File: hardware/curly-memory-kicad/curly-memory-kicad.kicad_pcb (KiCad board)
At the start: 4 copper layers, 30 x 100 mm, 84 parts, among them J101 Conn_01x06, J102 Conn_01x05, J103 Conn_01x05, J104 Conn_01x05, J105 Conn_01x05, J106 Conn_01x05, J401 Conn_02x05_Odd_Even, U101 MCP3008-I/SL, U102 ESP32-WROOM-32, U103 MCP4822-E/SN, U104 MCP4822-E/SN, U105 MCP42010-E/SL, U106 MCP42010-E/SL, U201 MCP6004, U301 MCP6004, U401 NCP1117-5.0_SOT223, U402 NCP1117-3.3_SOT223

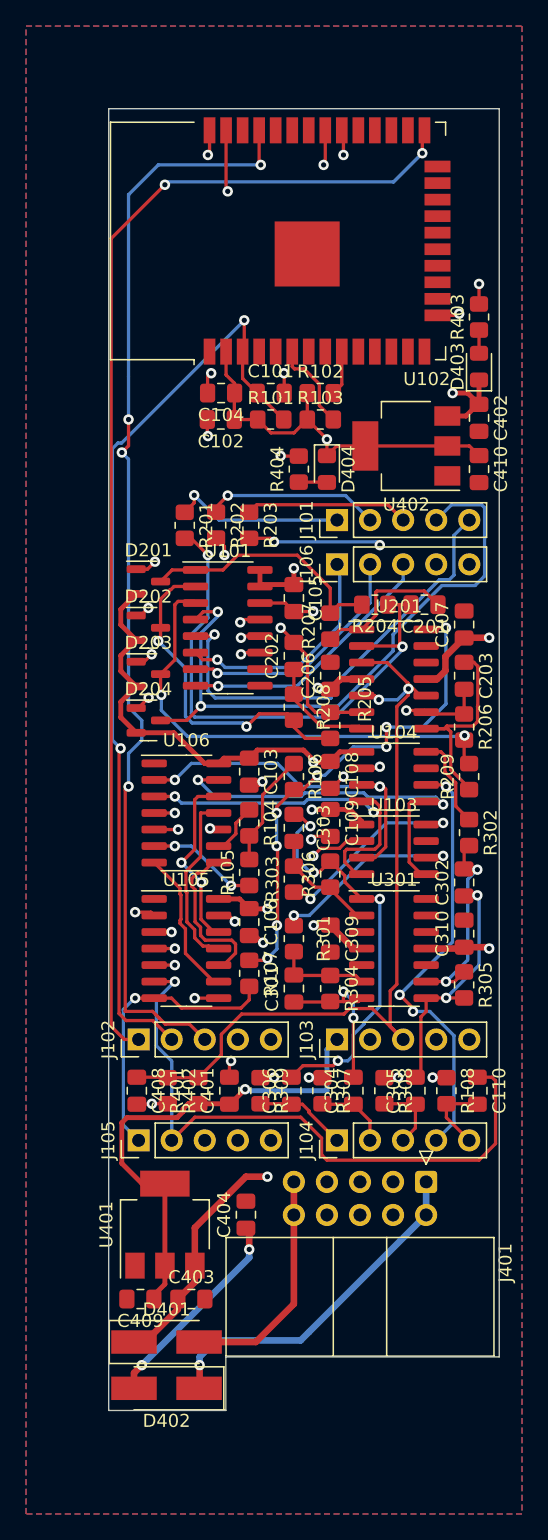
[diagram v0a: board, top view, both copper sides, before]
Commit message: more pcb tracked- again
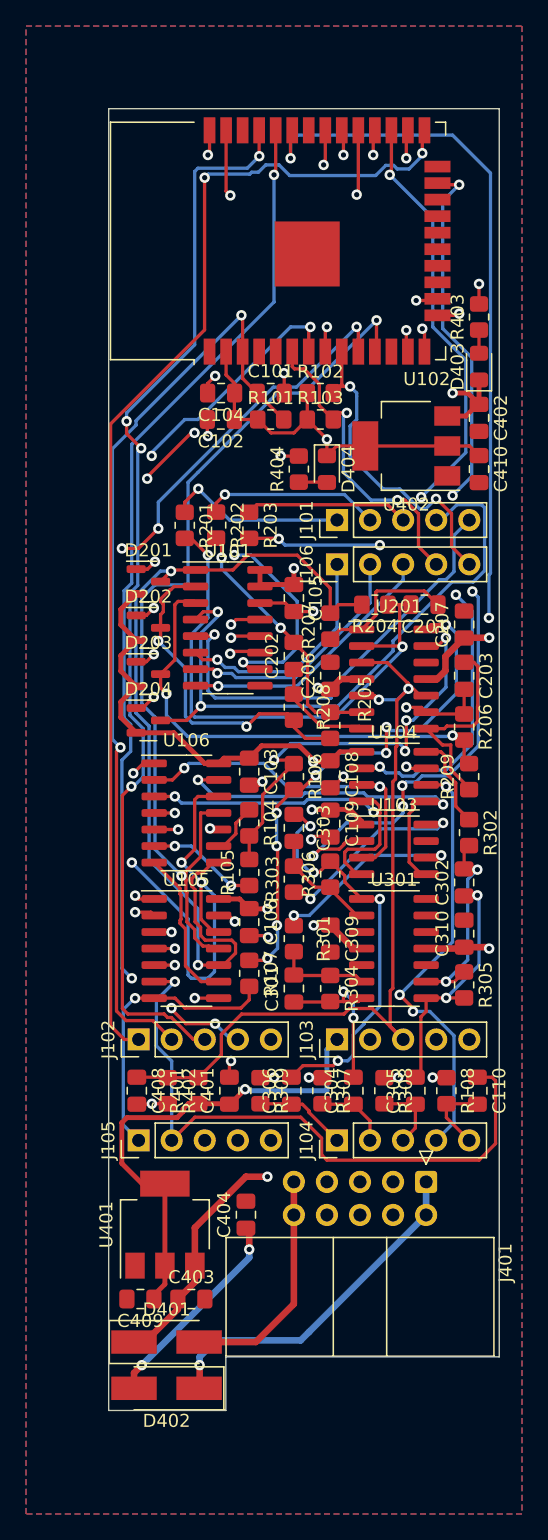
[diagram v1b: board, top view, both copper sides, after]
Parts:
- moved C109 0.05 mm to (17.0, 54.9)
- moved C108 0.05 mm to (17.0, 51.1)
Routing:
- net Net-(J103-Pad5): track 0.00 -> 87.9 mm, vias 0 -> 2
- net /PROG_RX: track 0.00 -> 81.2 mm, vias 0 -> 4
- net /SPI3_CS_1: track 0.00 -> 78.5 mm, vias 0 -> 2
- net /LEDS: track 0.00 -> 77.4 mm, vias 0 -> 2
- net /RES_~SHDN: track 14.0 -> 88.1 mm, vias 2 -> 6
- net Net-(J103-Pad4): track 0.00 -> 69.7 mm, vias 0 -> 1
- net /SPI2_CS_0: track 4.92 -> 69.4 mm, vias 1 -> 6
- net /SPI2_CS_1: track 1.45 -> 63.2 mm, vias 1 -> 4
- net /SPI2_CS_2: track 0.00 -> 59.1 mm, vias 0 -> 4
- net /RES_~RS: track 13.3 -> 70.4 mm, vias 0 -> 2
- net /SPI2_MOSI: track 28.0 -> 81.7 mm, vias 2 -> 3
- net /SPI3_CS_0: track 0.00 -> 52.5 mm, vias 0 -> 3
- net /SPI2_MISO: track 30.4 -> 75.6 mm, vias 2 -> 3
- net /SPI2_CLK: track 27.5 -> 71.4 mm, vias 2 -> 3
- net /IN_0: track 32.1 -> 67.5 mm, vias 0 -> 2
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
